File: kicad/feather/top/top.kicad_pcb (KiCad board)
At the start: 2 copper layers, 52 x 24.8 mm, 14 parts, among them J1 Conn_01x12_Socket, J2 Conn_01x16_Socket, J3 Conn_01x03_Socket

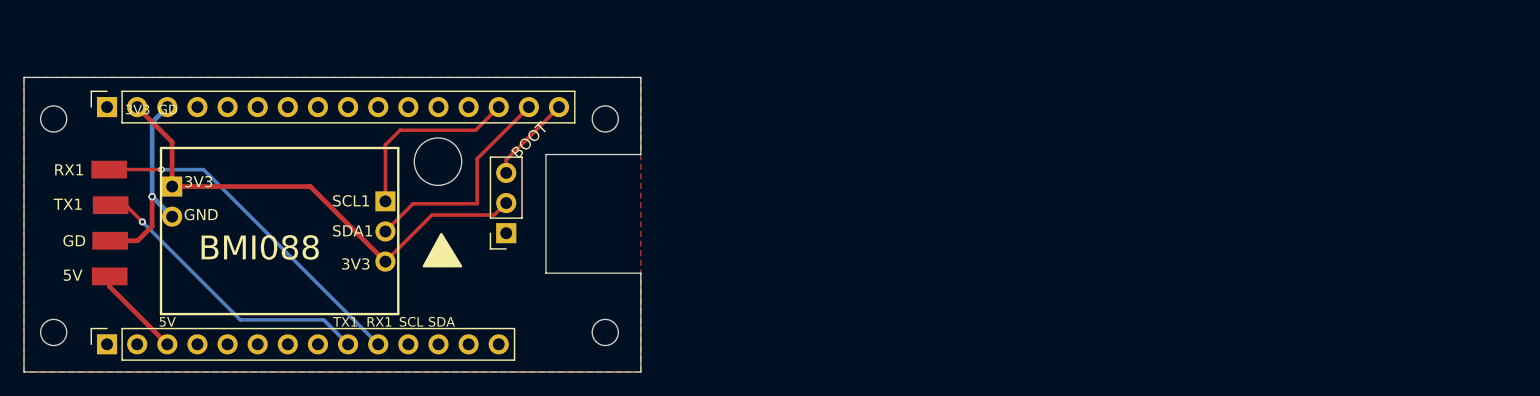
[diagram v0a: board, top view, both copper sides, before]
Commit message: modified:   kicad/feather/top/top.kicad_pro
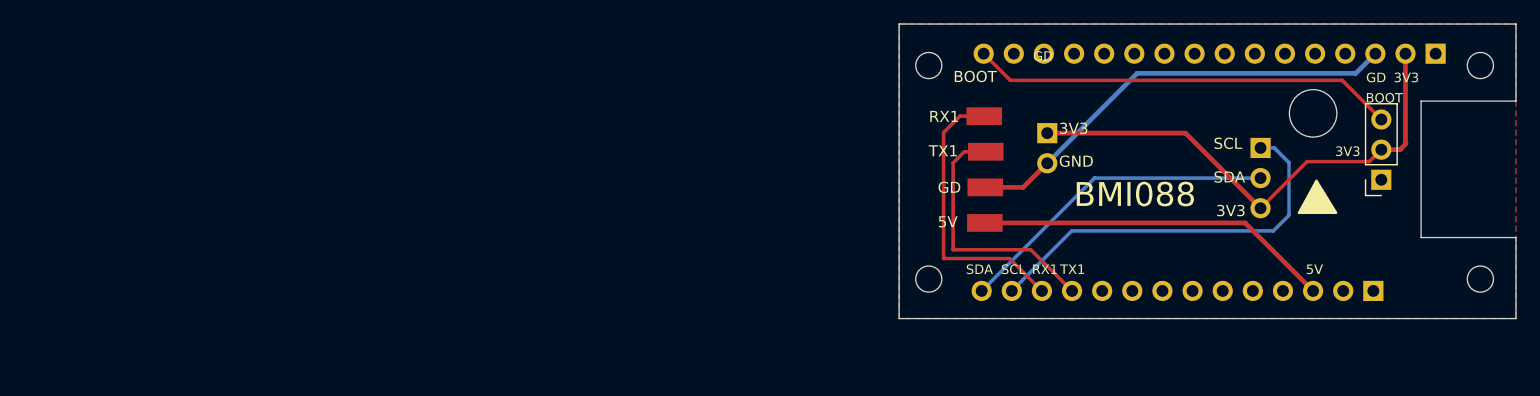
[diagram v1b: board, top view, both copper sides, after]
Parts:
- J1, J2: moved to B.Cu
- moved J2 112.1 mm to (182.0, 97.5)
- moved J1 106.8 mm to (176.8, 117.5)
- moved GND_PAD19 73.9 mm to (144.1, 111.9)
- moved GND_PAD21 73.9 mm to (144.1, 104.6)
- moved Motor5 73.9 mm to (166.5, 105.4)
- moved POST_2 73.9 mm to (138.9, 96.5)
- moved GND_PAD18 73.9 mm to (144.2, 110.2)
- moved GND_PAD20 73.9 mm to (144.2, 107.3)
- moved J3 73.9 mm to (177.4, 108.1)
- moved POST_3 73.9 mm to (185.8, 117.5)
- moved POST_4 73.9 mm to (139.7, 117.8)
- moved PMW3901_PWR2 73.9 mm to (152.3, 104.2)
- moved POST_1 73.9 mm to (187.1, 96.5)
- moved POST_5 73.9 mm to (171.7, 102.5)
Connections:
- J1 pad 10: /RX1 -> (no net)
- J1 pad 11: /SCL -> /TX1
- J1 pad 12: /SDA -> /RX1
- J1 pad 13: (no net) -> /SCL
- J1 pad 14: (no net) -> /SDA
- J1 pad 9: /TX1 -> (no net)
- Motor5 pad 1: /SCL1 -> /SCL
- Motor5 pad 2: /SDA1 -> /SDA
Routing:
- net /SCL: track 0.00 -> 33.4 mm
- net /BOOT: track 7.39 -> 35.8 mm
- net /SDA: track 0.00 -> 27.6 mm
- net /5V: track 7.74 -> 30.0 mm
- net /GND: track 17.0 -> 37.6 mm, vias 2 -> 0
- net /SDA1: track 18.8 -> 0.00 mm
- net /SCL1: track 15.7 -> 0.00 mm
- net /RX1: track 28.9 -> 24.0 mm, vias 2 -> 0
- net /TX1: track 24.9 -> 21.9 mm, vias 1 -> 0
- net /3V3: track 41.0 -> 43.0 mm
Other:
- outline, holes or cut-outs redrawn
- board text removed: "SCL1"
- board text removed: "SDA1"
